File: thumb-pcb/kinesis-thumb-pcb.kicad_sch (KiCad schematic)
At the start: 50 parts, among them J1 Conn_01x10, J2 Conn_01x10

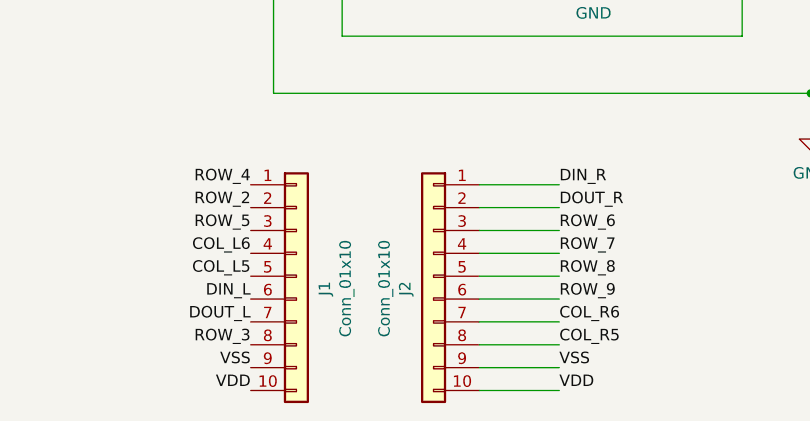
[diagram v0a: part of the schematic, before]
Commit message: Routed
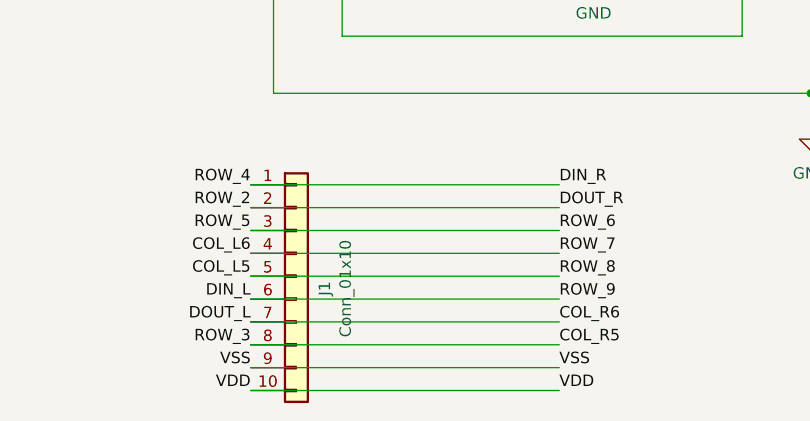
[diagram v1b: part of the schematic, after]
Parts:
- removed J2: Conn_01x10, Connector_PinHeader_2.54mm:PinHeader_1x10_P2.54mm_Vertical, symbol kicad_port-rescue:Conn_01x10-Connector_Generic
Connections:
- net DOUT_L is gone; now on net COL_R6: J1.7 (Pin_7), LED55.2 (DOUT)
- net ROW_2 is gone; now on net DOUT_R: D25.1 (K), J1.2 (Pin_2)
- net ROW_3 is gone; now on net COL_R5: D35.1 (K), D36.1 (K), J1.8 (Pin_8)
- net ROW_4 is gone; now on net DIN_R: D46.1 (K), J1.1 (Pin_1)
- net ROW_6 is gone; now on net ROW_5: D65.1 (K), D66.1 (K)
- net ROW_7 is gone; now on net COL_L6: D75.1 (K)
- net ROW_8 is gone; now on net COL_L5: D85.1 (K), D86.1 (K)
- net ROW_9 is gone; now on net DIN_L: D96.1 (K)
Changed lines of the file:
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@@
 	(wire
 		(pts
-			(xy 96.52 160.02) (xy 105.41 160.02)
-		)
-		(stroke
-			(width 0)
-			(type default)
-		)
-	)
-	(wire
-		(pts
 			(xy 109.22 30.48) (xy 109.22 31.75)
 		)
@@
 	(wire
 		(pts
-			(xy 96.52 180.34) (xy 105.41 180.34)
+			(xy 71.12 177.8) (xy 105.41 177.8)
 		)
 		(stroke
@@
 	(wire
 		(pts
-			(xy 96.52 165.1) (xy 105.41 165.1)
+			(xy 209.55 20.32) (xy 209.55 22.86)
 		)
 		(stroke
@@
 	(wire
 		(pts
-			(xy 209.55 20.32) (xy 209.55 22.86)
+			(xy 88.9 60.96) (xy 93.98 60.96)
 		)
 		(stroke
@@
 	(wire
 		(pts
-			(xy 88.9 60.96) (xy 93.98 60.96)
+			(xy 237.49 114.3) (xy 237.49 124.46)
 		)
 		(stroke
@@
 	(wire
 		(pts
-			(xy 237.49 114.3) (xy 237.49 124.46)
+			(xy 71.12 172.72) (xy 105.41 172.72)
 		)
 		(stroke
@@
 	(wire
 		(pts
+			(xy 71.12 167.64) (xy 105.41 167.64)
+		)
+		(stroke
+			(width 0)
+			(type default)
+		)
+	)
+	(wire
+		(pts
 			(xy 237.49 50.8) (xy 237.49 60.96)
 		)
@@
 	(wire
 		(pts
-			(xy 254 20.32) (xy 254 53.34)
+			(xy 71.12 157.48) (xy 105.41 157.48)
 		)
 		(stroke
@@
 	(wire
 		(pts
-			(xy 96.52 172.72) (xy 105.41 172.72)
+			(xy 254 20.32) (xy 254 53.34)
 		)
 		(stroke
@@
 	(wire
 		(pts
-			(xy 96.52 177.8) (xy 105.41 177.8)
+			(xy 73.66 91.44) (xy 73.66 147.32)
 		)
 		(stroke
@@
 	(wire
 		(pts
-			(xy 73.66 91.44) (xy 73.66 147.32)
+			(xy 93.98 50.8) (xy 93.98 60.96)
 		)
 		(stroke
@@
 	(wire
 		(pts
-			(xy 93.98 50.8) (xy 93.98 60.96)
+			(xy 222.25 30.48) (xy 222.25 31.75)
 		)
 		(stroke
@@
 	(wire
 		(pts
-			(xy 96.52 170.18) (xy 105.41 170.18)
+			(xy 237.49 124.46) (xy 237.49 125.73)
 		)
 		(stroke
@@
 	(wire
 		(pts
-			(xy 222.25 30.48) (xy 222.25 31.75)
+			(xy 71.12 162.56) (xy 105.41 162.56)
 		)
 		(stroke
@@
 	(wire
 		(pts
-			(xy 237.49 124.46) (xy 237.49 125.73)
+			(xy 118.11 91.44) (xy 109.22 91.44)
 		)
 		(stroke
@@
 	(wire
 		(pts
-			(xy 118.11 91.44) (xy 109.22 91.44)
+			(xy 71.12 165.1) (xy 105.41 165.1)
 		)
 		(stroke
@@
 	(wire
 		(pts
-			(xy 156.21 86.995) (xy 175.26 86.995)
+			(xy 71.12 180.34) (xy 105.41 180.34)
 		)
 		(stroke
@@
 	(wire
 		(pts
-			(xy 96.52 167.64) (xy 105.41 167.64)
+			(xy 156.21 86.995) (xy 175.26 86.995)
 		)
 		(stroke
@@
 	(wire
 		(pts
+			(xy 71.12 175.26) (xy 105.41 175.26)
+		)
+		(stroke
+			(width 0)
+			(type default)
+		)
+	)
+	(wire
+		(pts
 			(xy 36.195 86.995) (xy 50.8 86.995)
 		)
@@
 	(wire
 		(pts
-			(xy 133.35 147.32) (xy 133.35 151.13)
+			(xy 71.12 170.18) (xy 105.41 170.18)
 		)
 		(stroke
@@
 	(wire
 		(pts
-			(xy 109.22 81.28) (xy 109.22 91.44)
+			(xy 133.35 147.32) (xy 133.35 151.13)
 		)
 		(stroke
@@
 	(wire
 		(pts
-			(xy 109.22 97.79) (xy 109.22 100.33)
+			(xy 109.22 81.28) (xy 109.22 91.44)
 		)
 		(stroke
@@
 	(wire
 		(pts
-			(xy 246.38 124.46) (xy 237.49 124.46)
+			(xy 109.22 97.79) (xy 109.22 100.33)
 		)
 		(stroke
@@
 	(wire
 		(pts
-			(xy 217.17 30.48) (xy 222.25 30.48)
+			(xy 246.38 124.46) (xy 237.49 124.46)
 		)
 		(stroke
@@
 	(wire
 		(pts
-			(xy 217.17 60.96) (xy 222.25 60.96)
+			(xy 217.17 30.48) (xy 222.25 30.48)
 		)
 		(stroke
@@
 	(wire
 		(pts
-			(xy 118.11 30.48) (xy 109.22 30.48)
+			(xy 217.17 60.96) (xy 222.25 60.96)
 		)
 		(stroke
@@
 	(wire
 		(pts
-			(xy 96.52 175.26) (xy 105.41 175.26)
+			(xy 118.11 30.48) (xy 109.22 30.48)
 		)
 		(stroke
@@
 	(wire
 		(pts
-			(xy 96.52 162.56) (xy 105.41 162.56)
+			(xy 254 68.58) (xy 254 83.82)
 		)
 		(stroke
@@
 	(wire
 		(pts
-			(xy 254 68.58) (xy 254 83.82)
+			(xy 246.38 60.96) (xy 237.49 60.96)
 		)
 		(stroke
@@
 	(wire
 		(pts
-			(xy 246.38 60.96) (xy 237.49 60.96)
+			(xy 71.12 160.02) (xy 105.41 160.02)
 		)
 		(stroke
@@
 	(wire
 		(pts
-			(xy 96.52 157.48) (xy 105.41 157.48)
-		)
-		(stroke
-			(width 0)
-			(type default)
-		)
-	)
-	(wire
-		(pts
 			(xy 93.98 81.28) (xy 93.98 91.44)
 		)
@@
 					(unit 1)
 				)
-			)
-		)
-	)
-	(symbol
-		(lib_id "kicad_port-rescue:Conn_01x10-Connector_Generic")
-		(at 91.44 167.64 0)
-		(mirror y)
-		(unit 1)
-		(exclude_from_sim no)
-		(in_bom yes)
-		(on_board yes)
-		(dnp no)
-		(property "Reference" "J2"
-			(at 88.2904 169.0116 90)
-			(effects
-				(font
-					(size 1.27 1.27)
-				)
-			)
-		)
-		(property "Value" "Conn_01x10"
-			(at 85.979 169.0116 90)
-			(effects
-				(font
-					(size 1.27 1.27)
-				)
-			)
-		)
-		(property "Footprint" "Connector_PinHeader_2.54mm:PinHeader_1x10_P2.54mm_Vertical"
-			(at 91.44 167.64 0)
-			(effects
-				(font
-					(size 1.27 1.27)
-				)
-				(hide yes)
-			)
-		)
-		(property "Datasheet" "~"
-			(at 91.44 167.64 0)
-			(effects
-				(font
-					(size 1.27 1.27)
-				)
-				(hide yes)
-			)
-		)
-		(property "Description" ""
-			(at 91.44 167.64 0)
-			(effects
-				(font
-					(size 1.27 1.27)
-				)
-			)
-		)
-		(pin "1"
-		)
-		(pin "10"
-		)
-		(pin "2"
-		)
-		(pin "3"
-		)
-		(pin "4"
-		)
-		(pin "5"
-		)
-		(pin "6"
-		)
-		(pin "7"
-		)
-		(pin "8"
-		)
-		(pin "9"
-		)
-		(instances
-			(project "kinesis-thumb-pcb"
-				(path "/c801d42e-dd94-493e-bd2f-6c3ddad43f55"
-					(reference "J2")
-					(unit 1)
-				)
